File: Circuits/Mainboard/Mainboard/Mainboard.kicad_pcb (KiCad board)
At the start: 2 copper layers, 170 x 170 mm, 72 parts, among them IC1 LM74500QDDFRQ1, IC2 LM74500QDDFRQ1, IC3 2536030320001, IC4 SX1280IMLTRT, IC5 SKY66122-11, IC6 TS2596CM533_RNG, IC7 TPS563300DRLR, J1 XT60PW-M, J10 B5P-VH_LF__SN_, J11 B6B-PH-K-S, J12 B5P-VH_LF__SN_, J13 B6B-PH-K-S, J14 B5P-VH_LF__SN_, J15 SMA-J-P-H-RA-TH1, J16 B5P-VH_LF__SN_, J2 XT60PW-M, J22 61300211821, J23 61300211821, J24 61300211821, J25 Conn_01x06_Pin, J26 Conn_01x04_Pin, J3 Conn_01x06_Pin, J4 Conn_01x05_Pin, J5 B6B-PH-K-S, J6 B5P-VH_LF__SN_, J7 B6B-PH-K-S, J8 Conn_01x06_Pin, J9 61300211821, Q1 PSMN6R7-40MLDX, Q2 PSMN6R7-40MLDX, U1 NUCLEOH723ZG

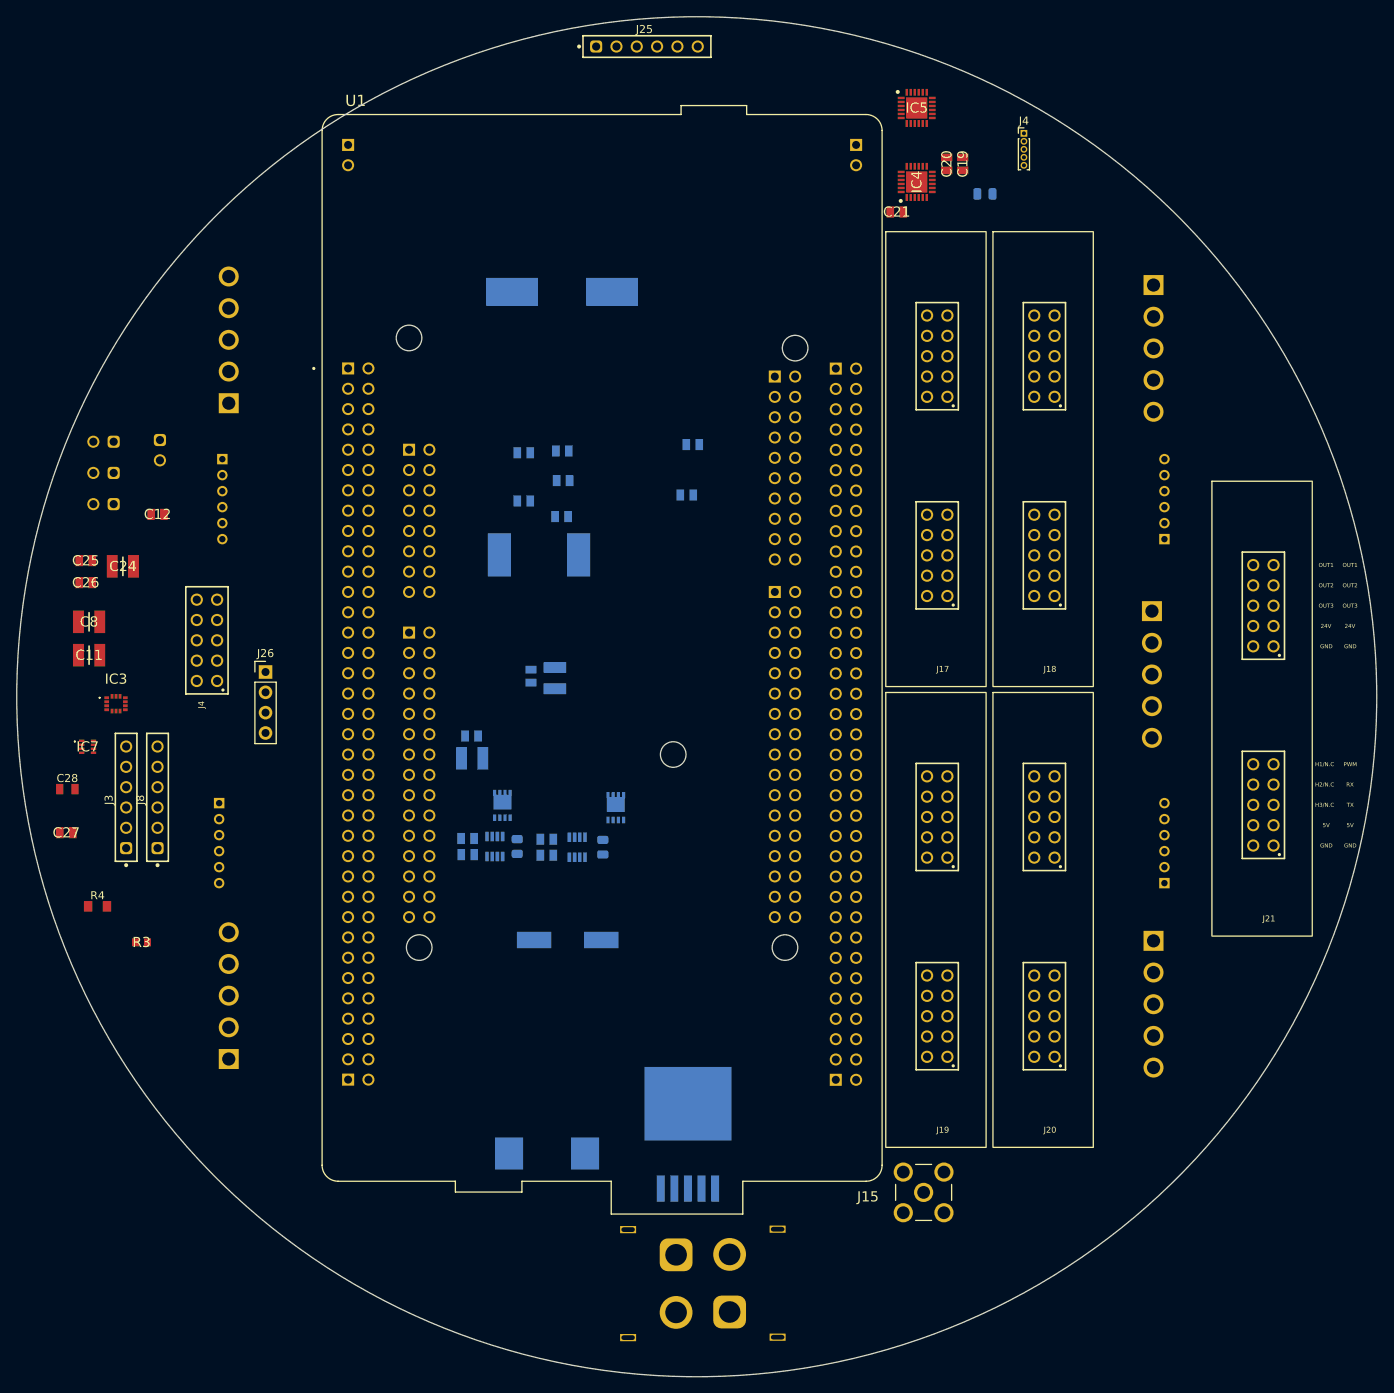
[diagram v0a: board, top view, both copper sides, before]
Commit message: Step file for mainboard pcb updated layout
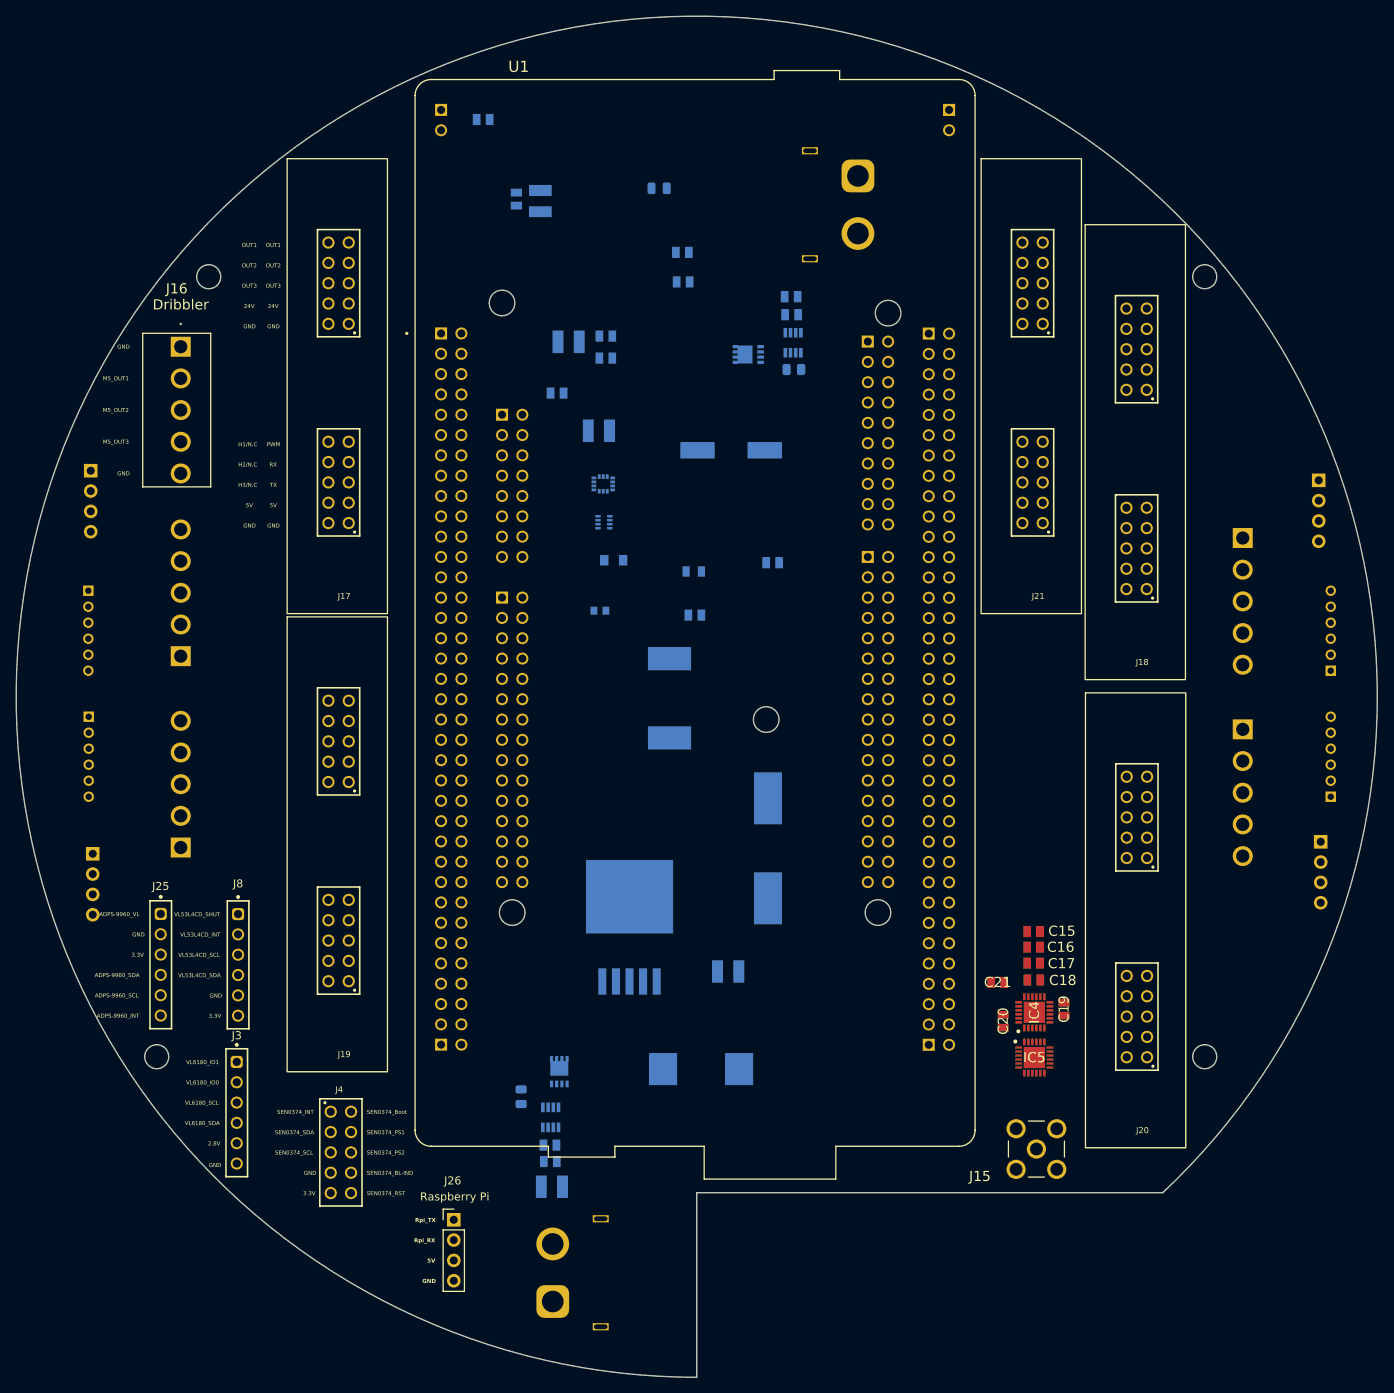
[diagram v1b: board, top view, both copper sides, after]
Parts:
- removed J24: 61300211821, Socket_header_6_pins_single_straight:61300211821
- removed the J4 at (227.4, 58.1)
- added J27: Conn_01x04_Pin, Connector_PinHeader_2.54mm:PinHeader_1x04_P2.54mm_Vertical, B.Cu at (264.5, 146.6)
- C11, C12, C24, C25, C26, C27, C28, C8, IC3, IC7, R3, R4: moved to B.Cu
- C15, C16, C17, C18, J16: moved to F.Cu
- J22, J23, J9: value 61300211821 -> Conn_01x04_Pin; footprint Socket_header_6_pins_single_straight:61300211821 -> Connector_PinHeader_2.54mm:PinHeader_1x04_P2.54mm_Vertical
- moved J9 144.9 mm to (264.2, 101.5), turned to 180 degrees
- moved J1 142.9 mm to (206.7, 63.4), turned to -90 degrees
- moved J25 129.9 mm to (119.5, 162.0), turned to -90 degrees
- moved J16 125.8 mm to (122.0, 84.8)
- moved IC5 119.6 mm to (228.7, 173.6)
- moved C20 107.4 mm to (224.8, 169.1)
- moved C19 106.4 mm to (232.4, 167.6), turned to -90 degrees
- moved IC4 104.8 mm to (228.7, 167.9)
- moved C21 97.1 mm to (224.1, 164.2)
- moved C11 88.1 mm to (168.4, 189.8), turned to 180 degrees
- moved C15 87.4 mm to (228.6, 157.8)
- moved C17 86.0 mm to (228.6, 161.8)
- moved C27 83.1 mm to (186.3, 118.3), turned to 180 degrees
- moved C28 82.9 mm to (186.1, 112.8), turned to 180 degrees
- moved R4 77.7 mm to (176.1, 111.5), turned to 180 degrees
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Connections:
- J11 pad 2: /5V_RF -> /5V
- J22 pad 1: /M2_Encoder_A -> /5V
- J22 pad 2: /M2_Encoder_B -> /M1_Encoder_A
- J23 pad 1: /M1_Encoder_A -> /5V
- J23 pad 2: /M1_Encoder_B -> /M3_Encoder_A
- J9 pad 1: /M4_Encoder_A -> /5V
- J9 pad 2: /M4_Encoder_B -> /M2_Encoder_A
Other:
- board size 170 x 170 mm -> 170.1 x 170.1 mm
- board text added: "2.8V"
- board text added: "3.3V"
- board text added: "ADPS-9960_INT"
- board text added: "ADPS-9960_SCL"
- board text added: "ADPS-9960_SDA"
- board text added: "ADPS-9960_VL"
- board text added: "Dribbler"
- board text added: "M1_H1"
- board text added: "M1_H2"
- board text added: "M1_H3"
- board text added: "M2_CH_A"
- board text added: "M2_CH_B"
- board text added: "M2_H1"
- board text added: "M2_H2"
- board text added: "M2_H3"
- board text added: "M3_H1"
- board text added: "M3_H2"
- board text added: "M3_H3"
- board text added: "M4_CH_A"
- board text added: "M4_CH_B"
- board text added: "M4_H1"
- board text added: "M4_H2"
- board text added: "M4_H3"
- board text added: "M5_OUT1"
- board text added: "M5_OUT2"
- board text added: "M5_OUT3"
- board text added: "Raspberry Pi"
- board text added: "Rpi_RX"
- board text added: "Rpi_TX"
- board text added: "SEN0374_BL-IND"
- board text added: "SEN0374_Boot"
- board text added: "SEN0374_INT"
- board text added: "SEN0374_PS1"
- board text added: "SEN0374_PS2"
- board text added: "SEN0374_RST"
- board text added: "SEN0374_SCL"
- board text added: "SEN0374_SDA"
- board text added: "VL53L4CD_INT"
- board text added: "VL53L4CD_SCL"
- board text added: "VL53L4CD_SDA"
- board text added: "VL53L4CD_SHUT"
- board text added: "VL6180_IO0"
- board text added: "VL6180_IO1"
- board text added: "VL6180_SCL"
- board text added: "VL6180_SDA"
